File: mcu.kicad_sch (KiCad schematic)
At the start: 13 parts, among them J2 Conn_2Rows-05Pins, U1 M24C02-RMN, U2 STM32C031C6Tx, Y1 8

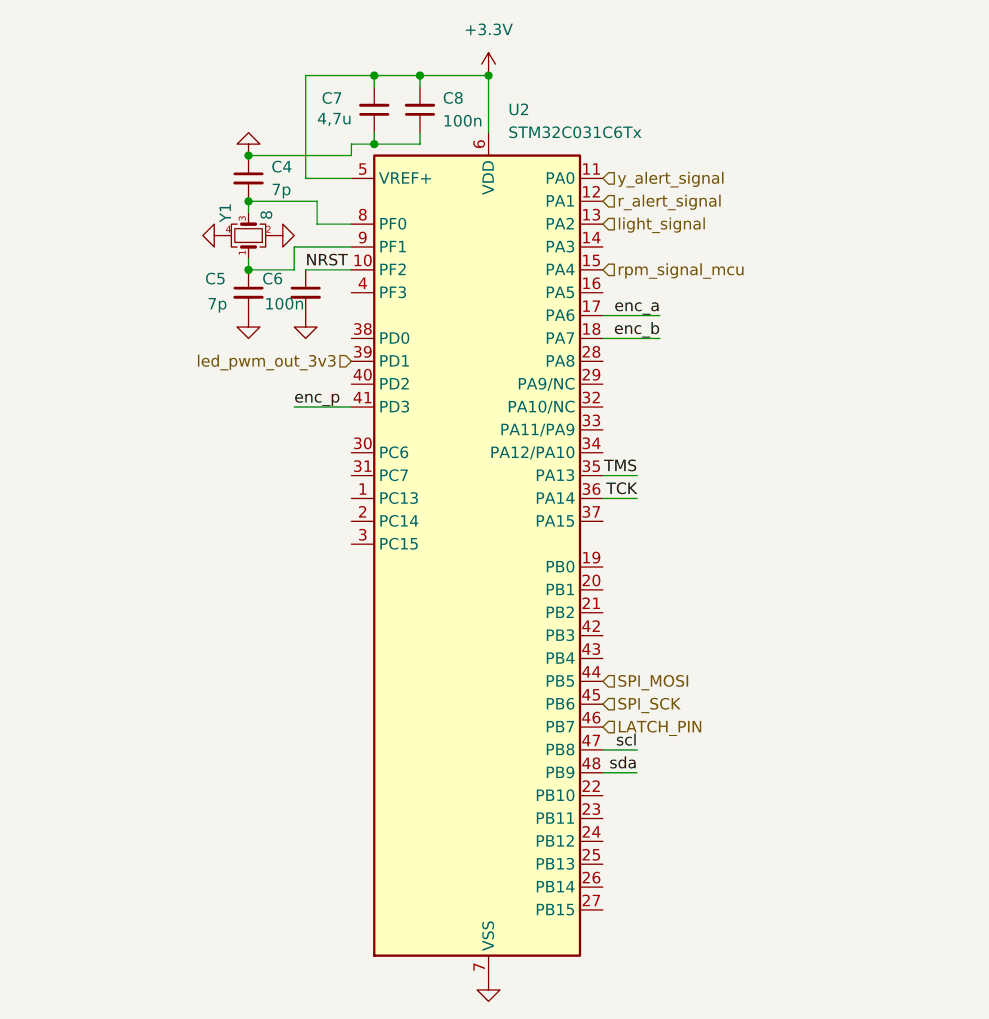
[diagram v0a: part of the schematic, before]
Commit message: stm32c031g6u6
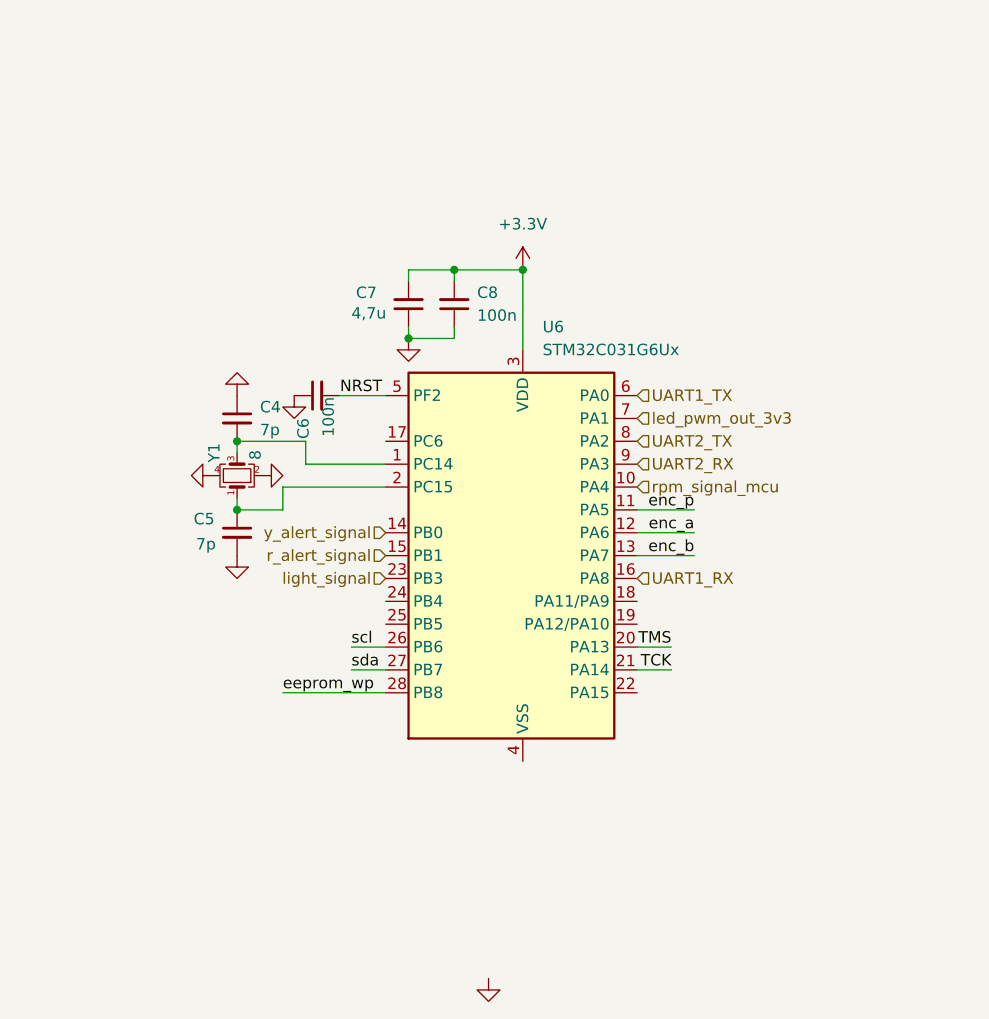
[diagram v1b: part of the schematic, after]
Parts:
- removed U2: STM32C031C6Tx, Package_QFP:LQFP-48_7x7mm_P0.5mm, symbol MCU_ST_STM32C0:STM32C031C6Tx
- added U6: STM32C031G6Ux, Library_local:QFN-28_4x4mm_P0.5mm, symbol MCU_ST_STM32C0:STM32C031G6Ux
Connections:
- net +3.3V: now also U6.3 (VDD)
- net ENCODER_A: now also U6.12 (PA6)
- net ENCODER_B: now also U6.13 (PA7)
- net ENCODER_BTN: now also U6.11 (PA5)
- net GND: now also C6.1; no longer C6.2
- net NRST: now also C6.2, U6.5 (PF2); no longer C6.1
- net TCK: now also U6.21 (PA14)
- net TMS: now also U6.20 (PA13)
- net eeprom_wp: now also U6.28 (PB8)
- net led_pwm_out_3v3: now also U6.7 (PA1)
- net light_signal: now also U6.23 (PB3)
- net r_alert_signal: now also U6.15 (PB1)
- net rpm_signal_mcu: now also U6.10 (PA4)
- net scl: now also U6.26 (PB6)
- net sda: now also U6.27 (PB7)
- net y_alert_signal: now also U6.14 (PB0)
- net at C5.1, Y1.1: now also U6.2 (PC15)
- net at C4.2, Y1.3: now also U6.1 (PC14)
- new net UART1_RX: U6.16 (PA8)
- new net UART1_TX: U6.6 (PA0)
- new net UART2_RX: U6.9 (PA3)
- new net UART2_TX: U6.8 (PA2)
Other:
- moved on the sheet: C4, C5, C6, C7, C8, Y1
